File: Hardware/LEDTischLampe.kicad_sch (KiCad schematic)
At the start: 39 parts, among them J1 Conn_01x02_Socket, J2 USB_C_Receptacle_USB2.0_14P, J3 Conn_02x03_Counter_Clockwise, Q1 P-CHANNEL-MOSFET, SW1 Reset, SW2 User, U1 ESP32-C3-WROOM-02, U7 RY8310

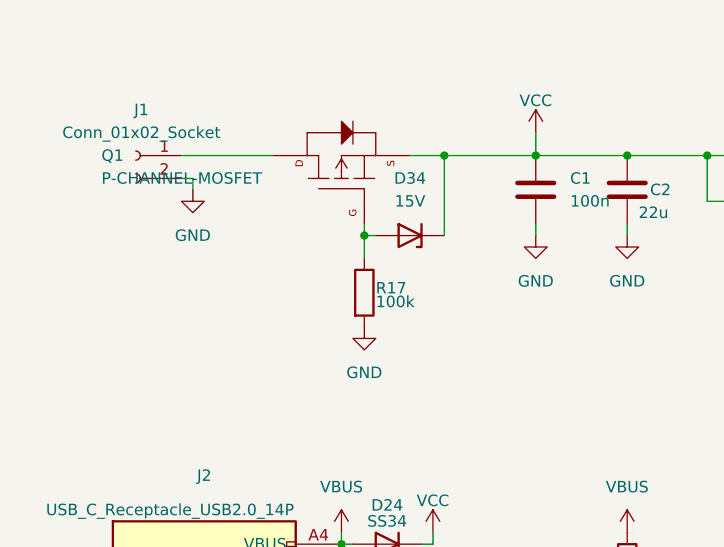
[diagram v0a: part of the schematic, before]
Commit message: final touches for v1.0
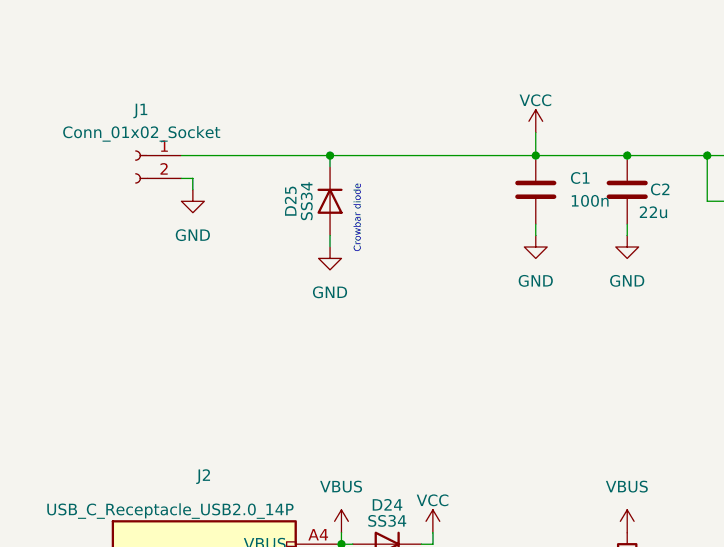
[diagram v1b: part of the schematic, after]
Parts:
- removed D34: 15V, Diode_SMD:D_0402_1005Metric, symbol Device:D_Zener
- removed Q1: P-CHANNEL-MOSFET, Package_SON:VSON-8_3.3x3.3mm_P0.65mm_NexFET, symbol Techbeard:P-CHANNEL-MOSFET
- removed R17: 100k, Resistor_SMD:R_0402_1005Metric, symbol Device:R
- added D25: SS34, Diode_SMD:D_SMA, symbol Device:D
- C1, C16, C25, C4, C5, C7, C8: LCSC C307331 -> (none)
- C18, C2, C6: footprint Capacitor_SMD:C_1210_3225Metric -> Capacitor_SMD:C_0805_2012Metric; LCSC C52306 -> (none)
- D1: LCSC C84256 -> (none)
- D2: LCSC C2296 -> (none)
- D24: LCSC C8678 -> (none)
- D3: LCSC C2297 -> (none)
- J2: LCSC C2927038 -> (none)
- L1: LCSC C5832376 -> (none)
- R1, R12, R13, R2, R20, R21, R3: LCSC C25900 -> (none)
- R10: LCSC C25792 -> (none)
- R11: LCSC C25756 -> (none)
- R14, R15: LCSC C25905 -> (none)
- SW1, SW2: LCSC C318884 -> (none)
- TH1: LCSC C2991699 -> (none)
- U1: LCSC C2934560 -> (none)
- U7: LCSC C370876 -> (none)
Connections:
- net GND: now also D25.2 (A)
- net VCC: now also J1.1 (Pin_1), D25.1 (K)
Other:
- note added: "Crowbar diode"
